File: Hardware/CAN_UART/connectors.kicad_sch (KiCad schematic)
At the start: 6 parts, among them J1 CAN, J2 Conn_02x23_Odd_Even, J3 Conn_02x23_Odd_Even, J4 UART

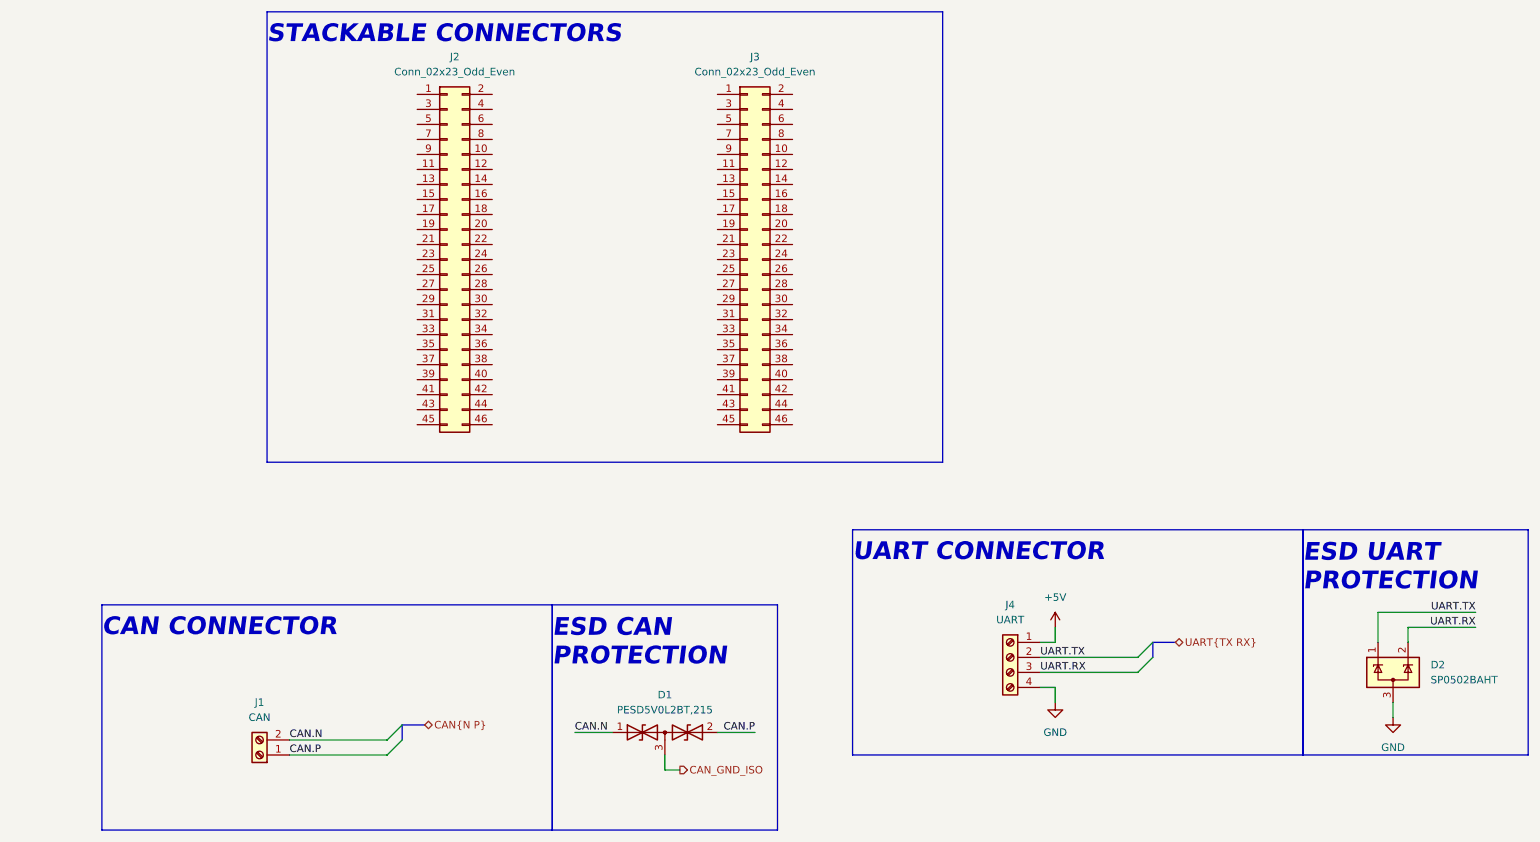
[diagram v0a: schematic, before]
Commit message: schematic update & pcb update
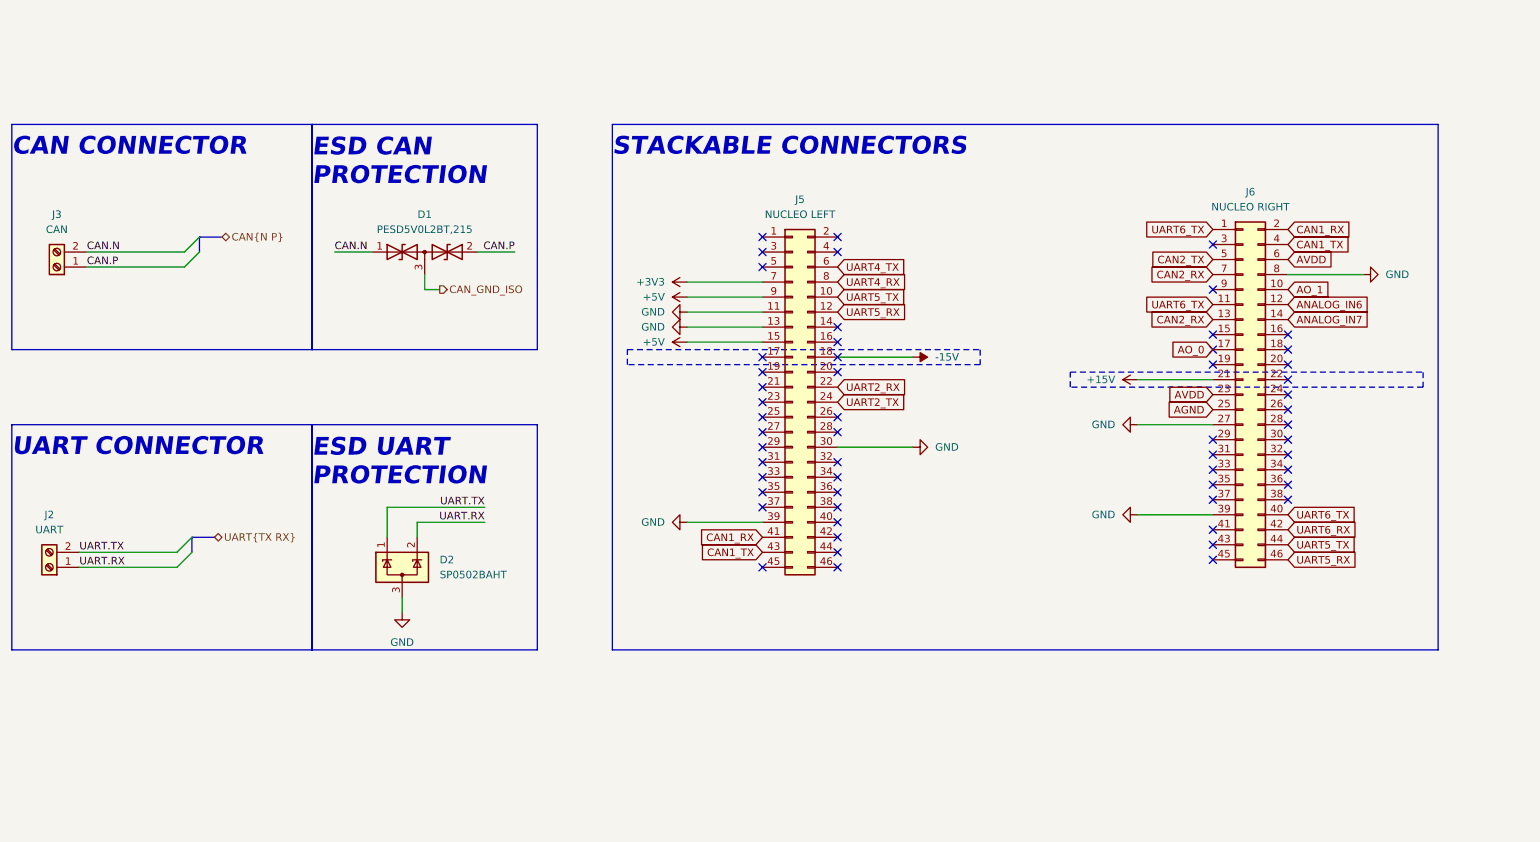
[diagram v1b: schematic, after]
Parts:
- removed J1: CAN, symbol Connector:Screw_Terminal_01x02
- removed J2, J3: Conn_02x23_Odd_Even, PLC_STM_Power:PRT12790, symbol Connector_Generic:Conn_02x23_Odd_Even
- removed J4: UART, symbol Connector:Screw_Terminal_01x04
- added J2: UART, PLC_STM:1725656, symbol Connector:Screw_Terminal_01x02
- added J3: CAN, PLC_STM:1725656, symbol Connector:Screw_Terminal_01x02
- added J5: NUCLEO LEFT, PLC_STM:PRT12790, symbol Connector_Generic:Conn_02x23_Odd_Even
- added J6: NUCLEO RIGHT, PLC_STM:PRT12790, symbol Connector_Generic:Conn_02x23_Odd_Even
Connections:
- net +5V: now also J5.15 (Pin_15), J5.9 (Pin_9)
- net CAN.N: now also J3.2 (Pin_2)
- net CAN.P: now also J3.1 (Pin_1)
- net GND: now also J5.11 (Pin_11), J5.13 (Pin_13), J5.30 (Pin_30), J5.39 (Pin_39), J6.27 (Pin_27), J6.39 (Pin_39), J6.8 (Pin_8)
- net UART.RX: now also J2.1 (Pin_1)
- net UART.TX: now also J2.2 (Pin_2)
- new net +15V: J6.21 (Pin_21)
- new net +3V3: J5.7 (Pin_7)
- new net -15V: J5.18 (Pin_18)
- new net AGND: J6.25 (Pin_25)
- new net ANALOG_IN6: J6.12 (Pin_12)
- new net ANALOG_IN7: J6.14 (Pin_14)
- new net AO_0: J6.17 (Pin_17)
- new net AO_1: J6.10 (Pin_10)
- new net AVDD: J6.23 (Pin_23), J6.6 (Pin_6)
- new net CAN1_RX: J5.41 (Pin_41), J6.2 (Pin_2)
- new net CAN1_TX: J5.43 (Pin_43), J6.4 (Pin_4)
- new net CAN2_RX: J6.13 (Pin_13), J6.7 (Pin_7)
- new net CAN2_TX: J6.5 (Pin_5)
- new net UART2_RX: J5.22 (Pin_22)
- new net UART2_TX: J5.24 (Pin_24)
- new net UART4_RX: J5.8 (Pin_8)
- new net UART4_TX: J5.6 (Pin_6)
- new net UART5_RX: J5.12 (Pin_12), J6.46 (Pin_46)
- new net UART5_TX: J5.10 (Pin_10), J6.44 (Pin_44)
- new net UART6_RX: J6.42 (Pin_42)
- new net UART6_TX: J6.1 (Pin_1), J6.11 (Pin_11), J6.40 (Pin_40)
- no-connect marks 0 -> 56
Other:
- moved on the sheet: D1, D2
